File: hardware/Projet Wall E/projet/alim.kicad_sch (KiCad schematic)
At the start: 42 parts, among them J201 USB_C_Receptacle_USB2.0_16P, J202 Conn_01x02, Q201 2SK3019, Q202 MMDT5401, Q203 DMP3099L, U201 AP2112K-3.3, U202 BQ27220YZFR, U203 USBLC6-2SC6, U204 BQ25896RTW

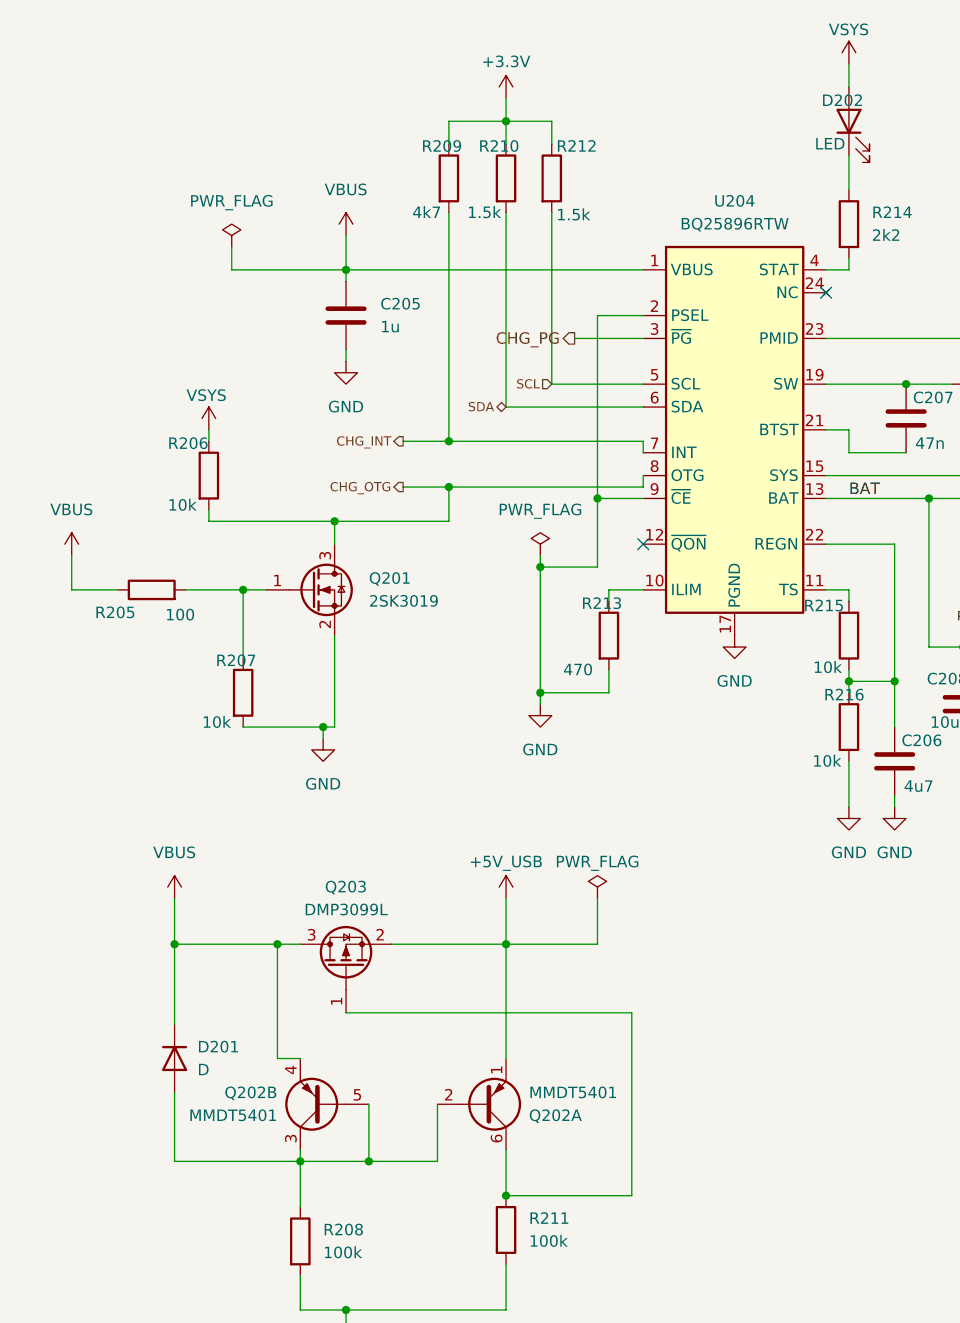
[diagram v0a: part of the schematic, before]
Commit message: Modifs schématique
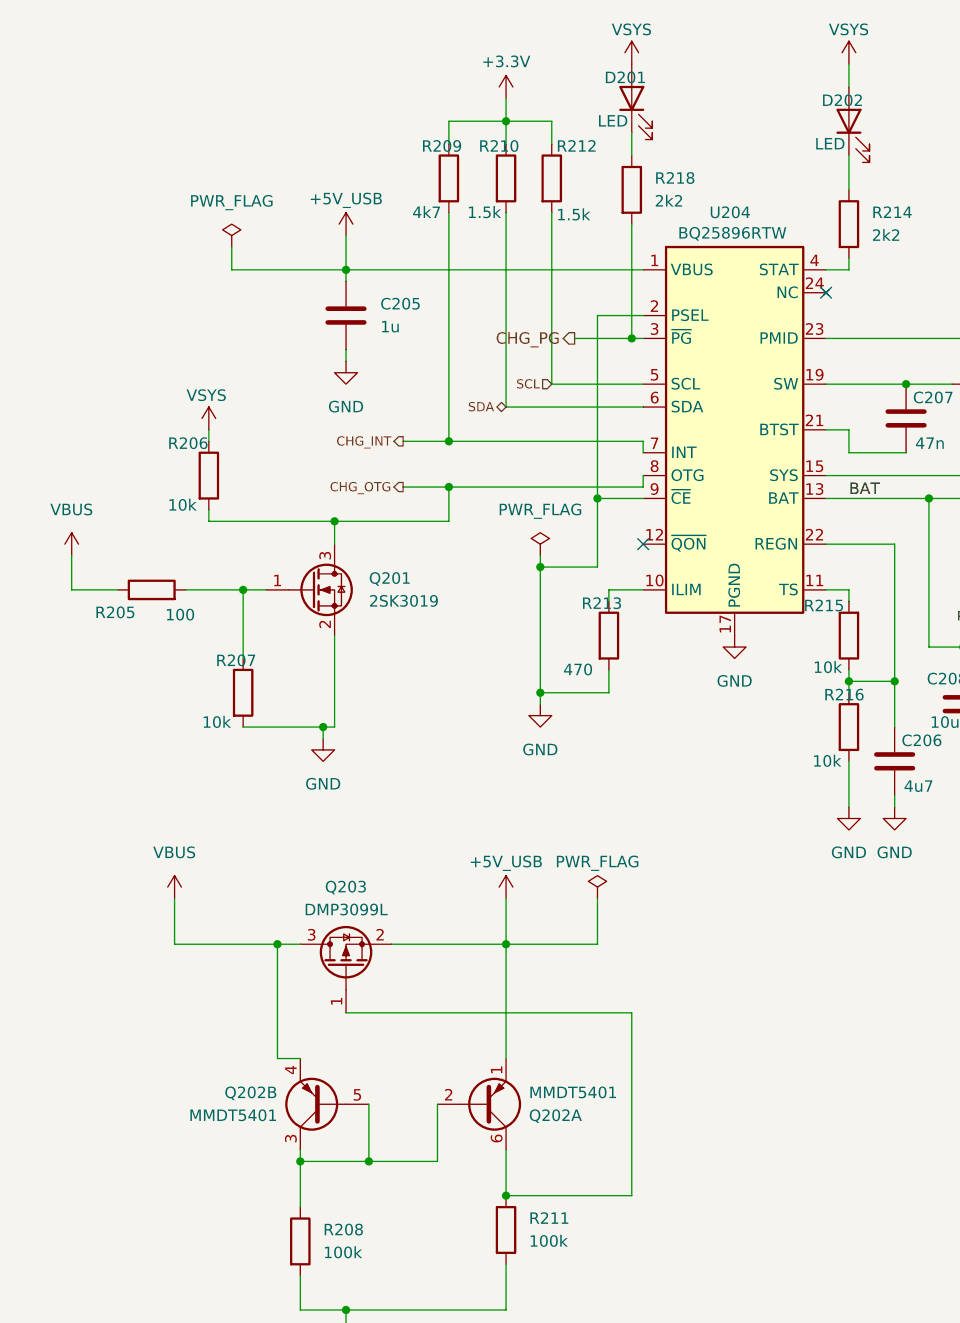
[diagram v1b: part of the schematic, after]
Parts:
- removed D201: D, Diode_SMD:D_SOD-523, symbol Device:D
- added D201: LED, LED_SMD:LED_0201_0603Metric, symbol wall_e:LED
- added R218: 2k2, Resistor_SMD:R_0402_1005Metric, symbol wall_e:R
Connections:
- net +5V_USB: now also C205.1, U204.1 (VBUS)
- net CHG_PG: now also R218.2
- net VBUS: no longer C205.1, U204.1 (VBUS)
- net VSYS: now also D201.2 (A)
- new net: D201.1 (K), R218.1
